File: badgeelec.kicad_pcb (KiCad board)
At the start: 2 copper layers, 44.9 x 43.2 mm, 34 parts, among them J1 PROG_CONN, U1 PIC16F716-I-SO-ND, U2 TSSP58038, Y1 4Mhz

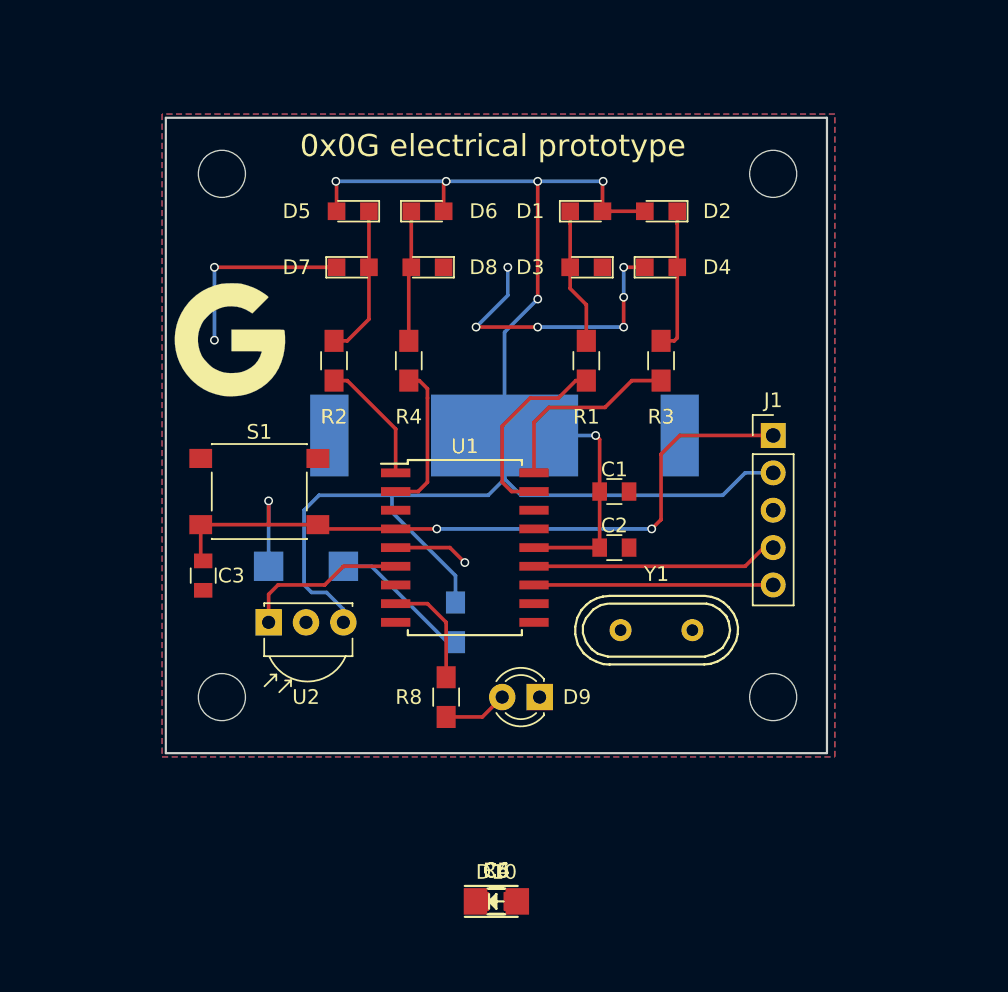
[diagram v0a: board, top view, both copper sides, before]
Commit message: Implemented prototypev2
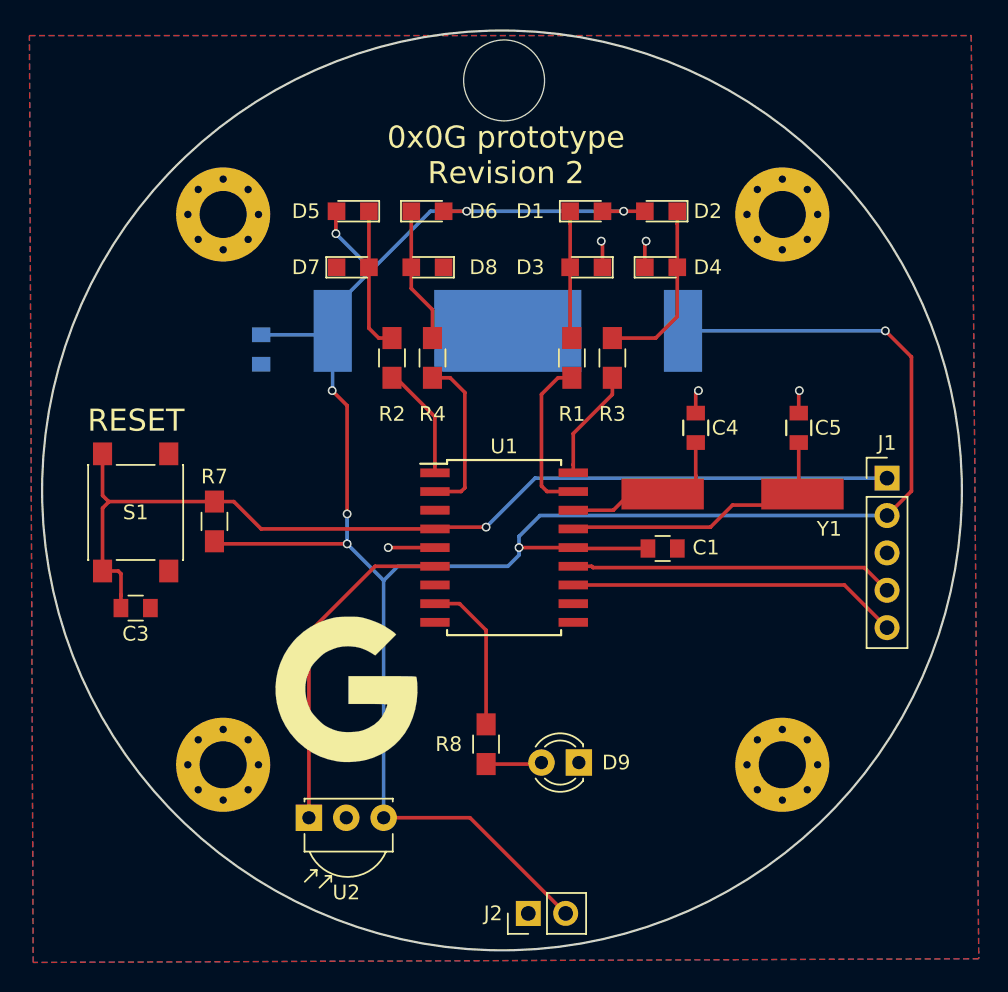
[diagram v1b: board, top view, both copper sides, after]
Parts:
- removed D10: LED, LEDs:LED_1206
- removed the G*** at (133.2, 90.0)
- removed JP1: permit operation / !program, Oddities:NetTie-I_SMD
- removed R6: 220, Resistors_SMD:R_0805_HandSoldering
- removed the REF** at (170.2, 78.7)
- removed the REF** at (170.2, 114.3)
- removed the REF** at (132.7, 78.7)
- removed the REF** at (132.7, 114.3)
- added G***: LOGO, 0gbadge-2018:g22ml_small, F.Cu at (141.2, 113.8)
- added J2: PWR_CONN, Pin_Headers:Pin_Header_Straight_1x02_Pitch2.54mm, F.Cu at (153.5, 129.0)
- added REF**: MountingHole_5.5mm, Mounting_Holes:MountingHole_5.5mm, F.Cu at (151.9, 72.4)
- added REF**: MountingHole_3.2mm_M3_Pad_Via, Mounting_Holes:MountingHole_3.2mm_M3_Pad_Via, F.Cu at (170.8, 118.9)
- added REF**: MountingHole_3.2mm_M3_Pad_Via, Mounting_Holes:MountingHole_3.2mm_M3_Pad_Via, F.Cu at (132.8, 118.9)
- added REF**: MountingHole_3.2mm_M3_Pad_Via, Mounting_Holes:MountingHole_3.2mm_M3_Pad_Via, F.Cu at (170.8, 81.5)
- added REF**: MountingHole_3.2mm_M3_Pad_Via, Mounting_Holes:MountingHole_3.2mm_M3_Pad_Via, F.Cu at (132.8, 81.5)
- C2: value 4.7uF -> 1uF; moved to B.Cu
- C3: value 100nF -> 10nF
- R7: value 1K -> 33K; moved to F.Cu
- Y1: footprint Crystals:Crystal_HC49-U_Vertical -> 0gbadge-2018:ABLS-4MHZ-B2-T
- moved C5 38.2 mm to (171.9, 96.0), turned to 90 degrees
- moved C4 34.9 mm to (164.9, 96.0), turned to 90 degrees
- moved C2 27.5 mm to (135.4, 90.7), turned to 270 degrees
- moved R7 17.8 mm to (132.2, 102.4), turned to 90 degrees
- moved U2 13.6 mm to (138.6, 122.5)
- moved Y1 10.6 mm to (167.4, 100.5)
- moved S1 8.52 mm to (126.9, 101.8), turned to 270 degrees
- moved J1 8.26 mm to (177.9, 99.4)
- moved BT1 7.12 mm to (152.1, 89.4)
- moved D9 5.19 mm to (157.0, 118.8)
- moved C3 5.09 mm to (126.9, 108.2), turned to 0 degrees
- moved C1 5.07 mm to (162.7, 104.2)
- moved R8 4.19 mm to (150.7, 117.5)
- moved R2 3.94 mm to (144.3, 91.2)
- moved R3 3.32 mm to (159.2, 91.2)
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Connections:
- R7 pad 2: Net-(JP1-Pad2) -> /~MCLR
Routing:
- net VDD: track 122.0 -> 170.5 mm, vias 6 -> 8
- net GND: track 38.9 -> 9.95 mm, vias 9 -> 5
- net Net-(C5-Pad1): track 0.00 -> 20.2 mm
- net /~MCLR: track 52.9 -> 67.1 mm, vias 3 -> 1
- net Net-(U1-Pad6): track 11.3 -> 23.0 mm
- net Net-(C4-Pad1): track 0.00 -> 11.2 mm
- net Net-(JP1-Pad2): track 9.76 -> 0.00 mm
- net /RB6: track 16.3 -> 22.5 mm
- net /RA1: track 13.2 -> 7.56 mm
- net /RB7: track 16.8 -> 22.0 mm
- net /RB2: track 7.69 -> 10.6 mm
- net Net-(D2-Pad1): track 9.79 -> 12.2 mm
- net /RA0: track 13.2 -> 11.1 mm
- net /RA3: track 10.3 -> 11.2 mm
- net /RA2: track 8.53 -> 7.83 mm
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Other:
- board size 44.9 x 43.2 mm -> 62.5 x 62.5 mm
- board text added: "0x0G prototype Revision 2"
- board text added: "RESET"
- board text removed: "0x0G electrical prototype"
- board text removed: "r1"
